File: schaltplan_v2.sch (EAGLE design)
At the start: 43 parts, among them T1 2N3565, T2 2N3565, T3 2N3565, T4 2N3565, T5 2N3565, T6 2N3565, T7 2N3565, T8 2N3565

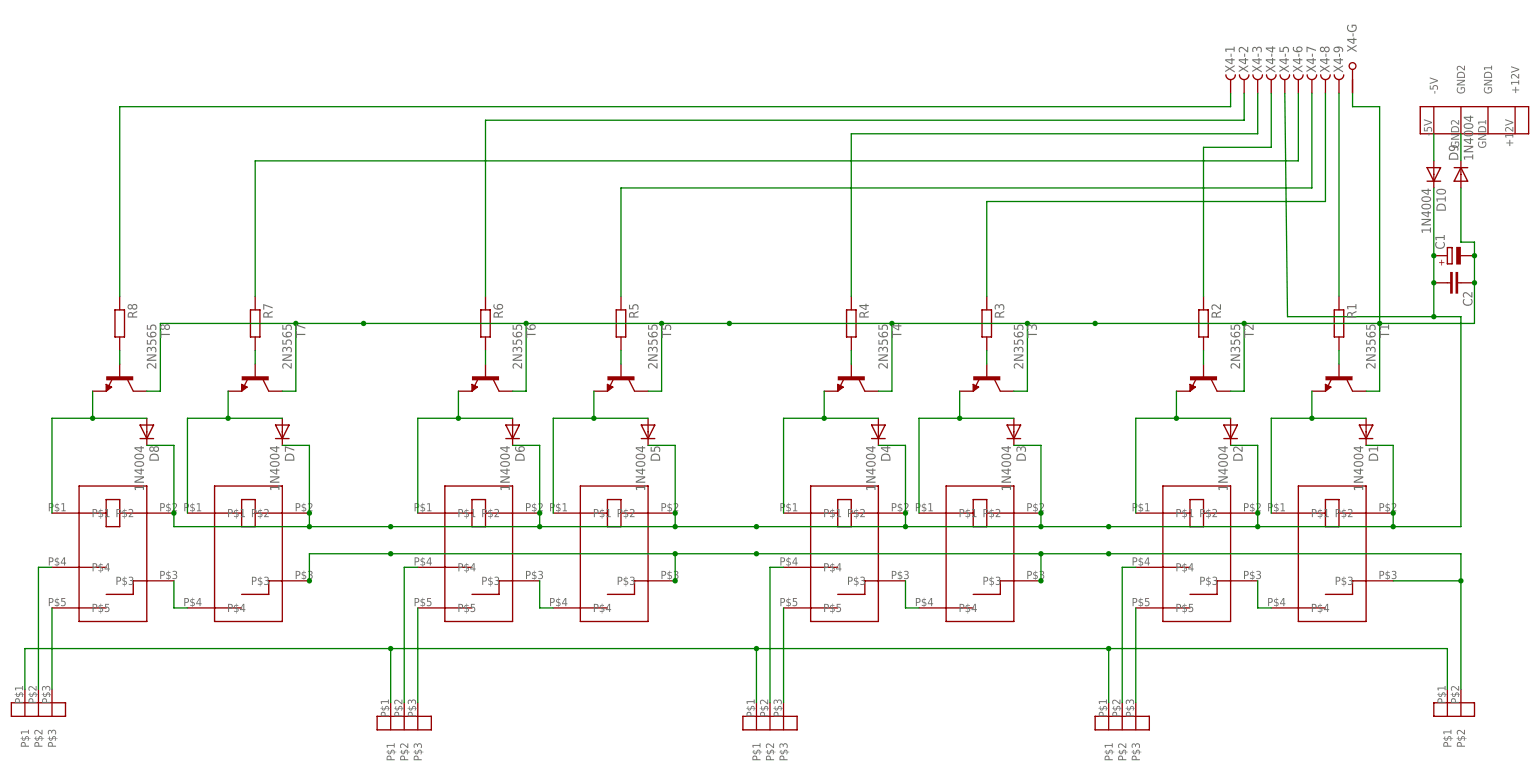
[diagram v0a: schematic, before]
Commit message: more layout fixes
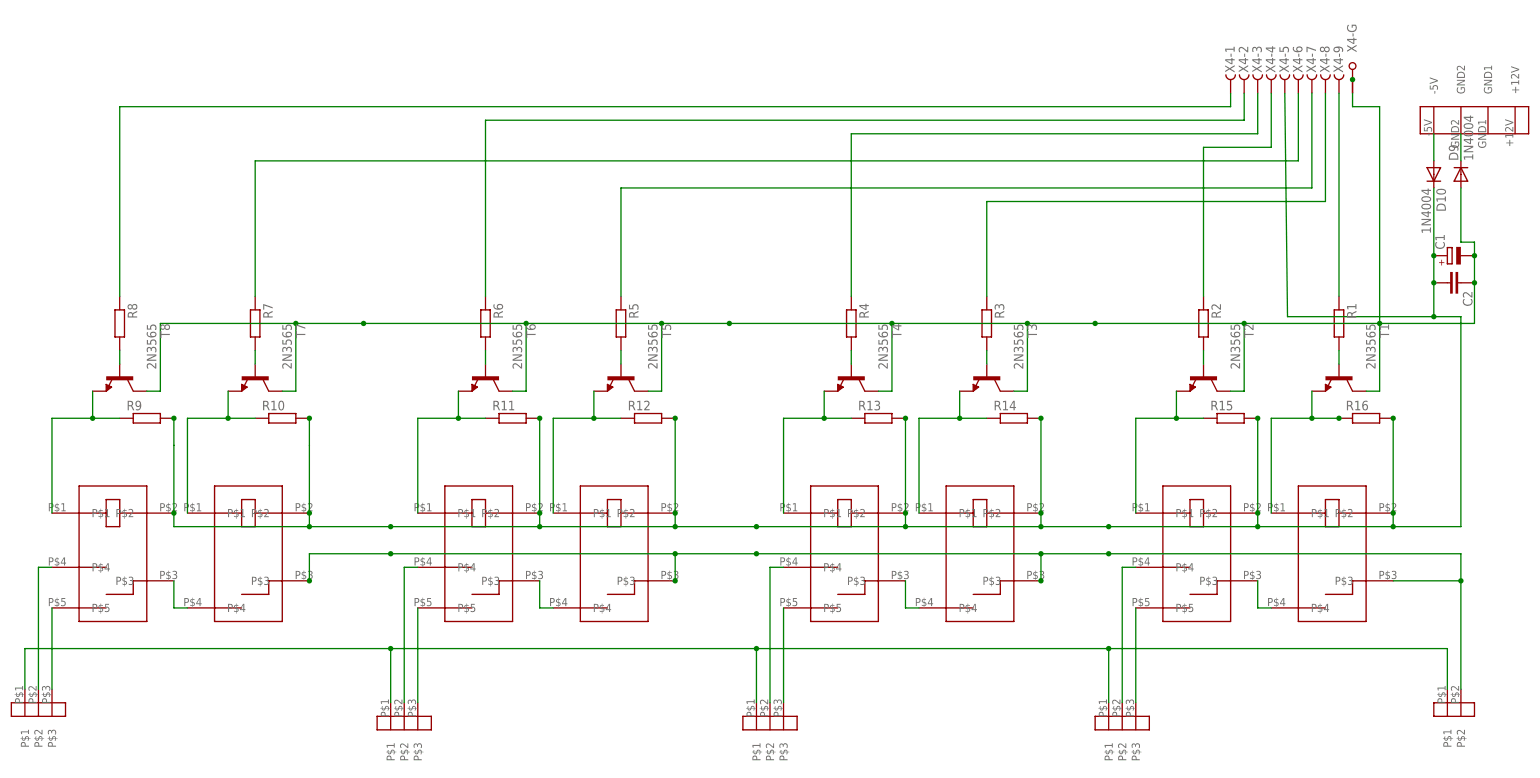
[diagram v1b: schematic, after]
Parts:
- removed D1, D2, D3, D4, D5, D6, D7, D8: 1N4004, diode:1N4004
- added R10, R11, R12, R13, R14, R15, R16, R9: (no value), rcl:R-EU_0207/2V
- R1, R2, R3, R4, R5, R6, R7, R8: device resistor:R-EU_0204/2V -> rcl:R-EU_0207/7
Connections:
- new net N$10: X4-G.G2
- net N$12: now also R15.1; no longer D2.A
- net N$20: now also R14.1; no longer D3.A
- net N$24: now also R10.2, R11.2, R12.2, R13.2, R14.2, R15.2, R16.2, R9.2; no longer D1.C, D2.C, D3.C, D4.C, D5.C, D6.C, D7.C, D8.C
- net N$25: now also R13.1; no longer D4.A
- net N$34: now also R12.1; no longer D5.A
- net N$39: now also R11.1; no longer D6.A
- net N$46: now also R10.1; no longer D7.A
- net N$51: now also R9.1; no longer D8.A
- net N$6: now also R16.1; no longer D1.A
